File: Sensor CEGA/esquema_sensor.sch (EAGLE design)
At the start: 11 parts

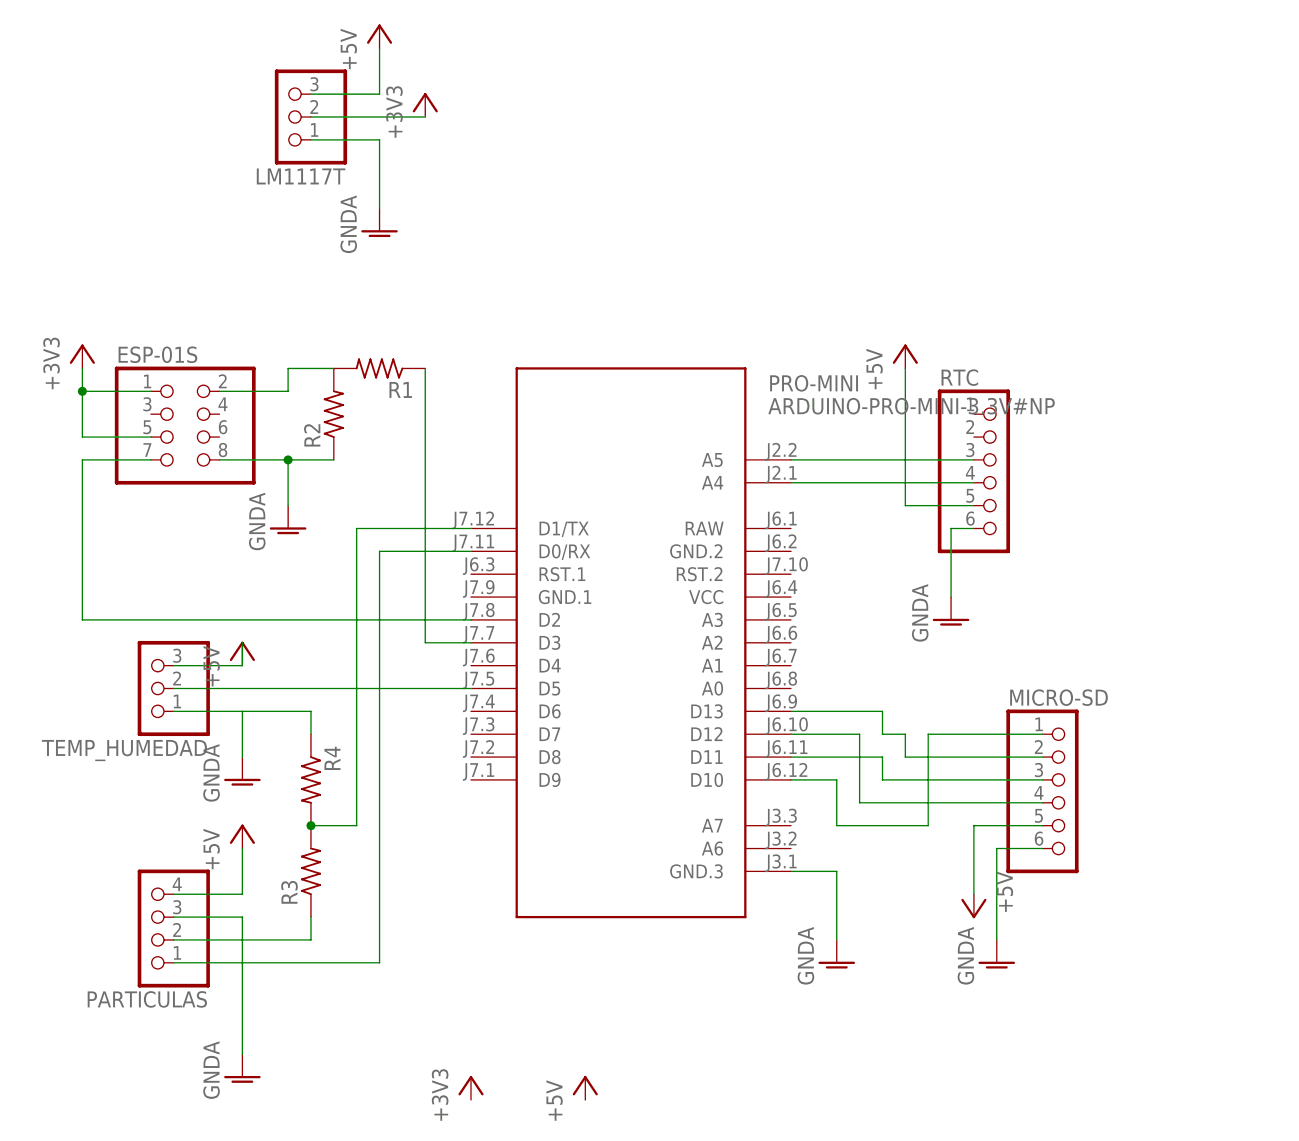
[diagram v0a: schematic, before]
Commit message: sensor cega v1, falta rutear las pistas
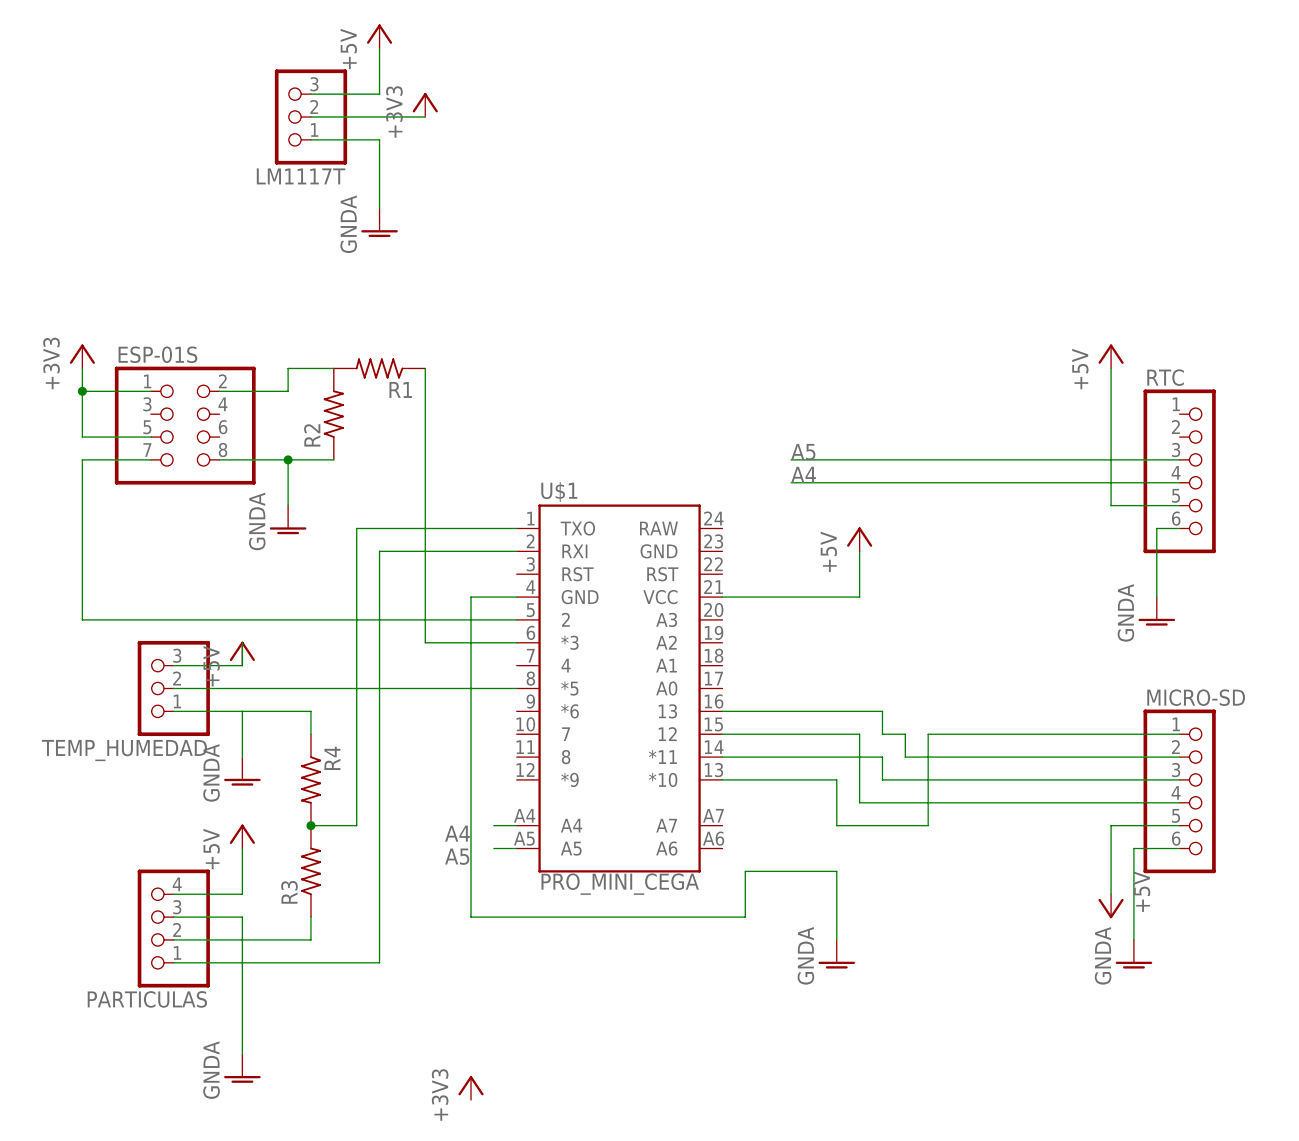
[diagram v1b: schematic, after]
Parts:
- removed PRO-MINI: ARDUINO-PRO-MINI-3.3V#NP, diy-modules:ARDUINO-PRO-MINI-3.3V#NP
- added U$1: PRO_MINI_CEGA, fablab_uchile:PRO_MINI_CEGA
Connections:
- removed net N$2: PRO-MINI.A4, RTC.4
- removed net N$9: PRO-MINI.A5, RTC.3
- new net A4: RTC.4, U$1.A4
- new net A5: RTC.3, U$1.A5
- net +5V: now also U$1.VCC
- net GNDA: now also U$1.GND; no longer PRO-MINI.GND.3
- net N$1: now also U$1.*3; no longer PRO-MINI.D3
- net N$10: now also U$1.12; no longer PRO-MINI.D12
- net N$11: now also U$1.*11; no longer PRO-MINI.D11
- net N$12: now also U$1.13; no longer PRO-MINI.D13
- net N$13: now also U$1.*10; no longer PRO-MINI.D10
- net N$3: now also U$1.2; no longer PRO-MINI.D2
- net N$5: now also U$1.RXI; no longer PRO-MINI.D0/RX
- net N$6: now also U$1.TXO; no longer PRO-MINI.D1/TX
- net N$8: now also U$1.*5; no longer PRO-MINI.D5
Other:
- moved on the sheet: MICRO-SD, RTC
